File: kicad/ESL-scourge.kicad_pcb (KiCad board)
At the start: 2 copper layers, 80 x 50 mm, 41 parts, among them IC1 MOC3020M, J1 DB9, J2 DB9, P1 CONN_4, P2 CONN_3, P3 CONN_4, Q1 BC847, Q2 BC847, Q3 BC847, U1 TDA2030

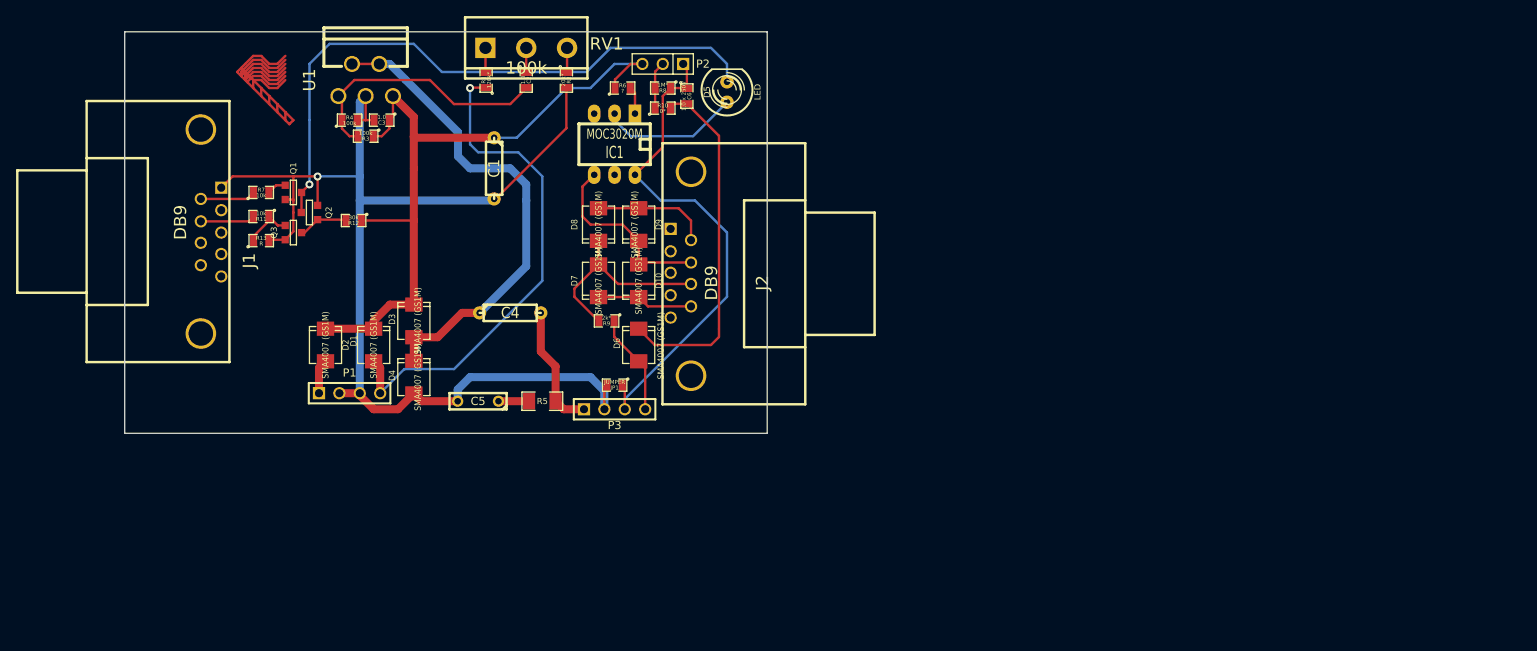
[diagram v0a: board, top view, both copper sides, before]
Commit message: Add initial maket_lovat as a separate branch (kicad folder only)
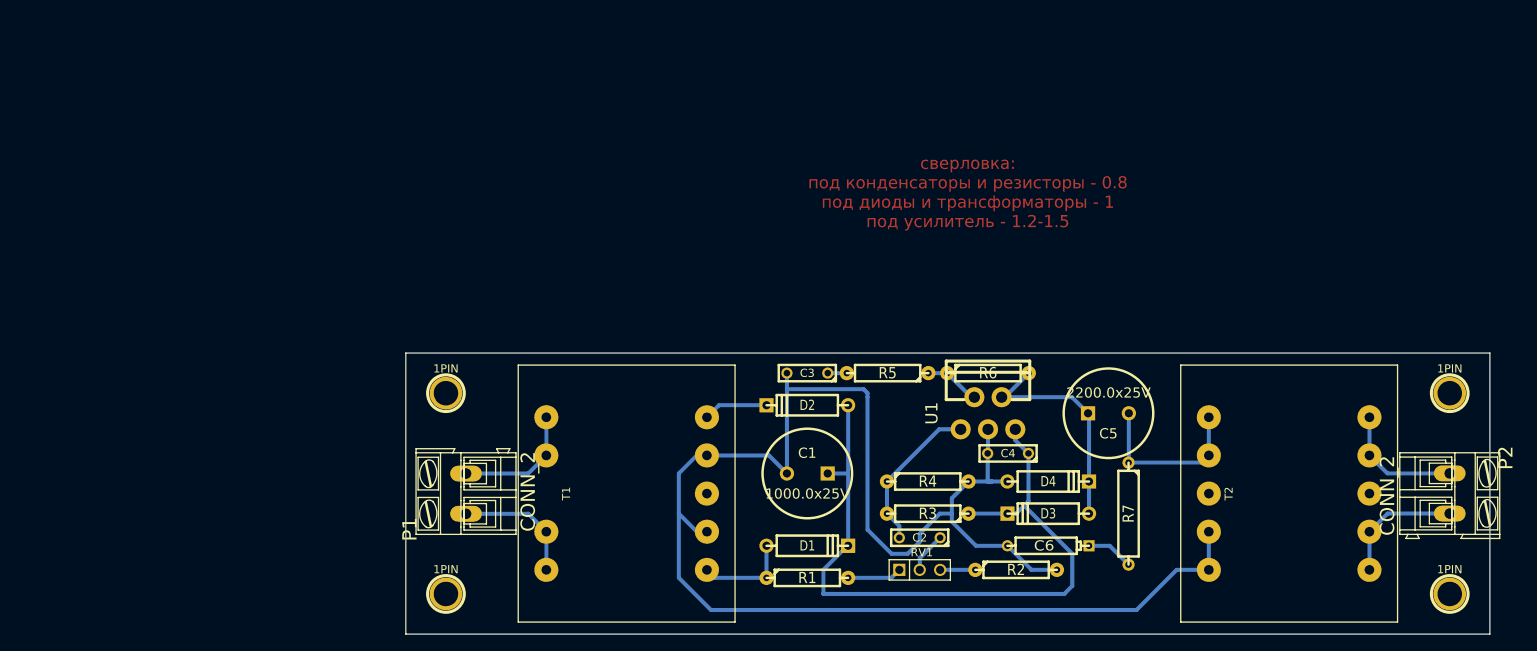
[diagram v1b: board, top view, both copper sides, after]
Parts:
- removed D10, D6, D7, D8, D9: SMA4007 (GS1M), DO_214AA
- removed D5: LED, LED-5MM
- removed IC1: MOC3020M, DIP-6__300_ELL
- removed J1: DB9, DB9MC
- removed J2: DB9, DB9FC
- removed JP1: JUMPER, SM0805
- removed P3: CONN_4, PIN_ARRAY_4x1
- removed Q1, Q2, Q3: BC847, SOT23EBC
- removed R10: 0*, SM0805
- removed R11: 10k, SM0805
- removed R12: 30k, SM0805
- removed R13: R, SM0805
- removed R8: 1M*, SM0805
- removed R9: 2k*, SM0805
- added 1PIN: P***, 1pin, F.Cu at (165.0, 45.0)
- added 1PIN: P***, 1pin, F.Cu at (165.0, 70.0)
- added 1PIN: P***, 1pin, F.Cu at (40.0, 45.0)
- added 1PIN: P***, 1pin, F.Cu at (40.0, 70.0)
- added T1: ТПК-1 (2х9В, 0.08А) (ТПГ-1), TPG-1, F.Cu at (62.5, 57.5)
- added T2: ТПК-1 (18В, 0.08А) (ТПГ-1), TPG-1, F.Cu at (145.0, 57.5)
- C1: footprint R3-LARGE_PADS -> C2V10
- C2, C3: footprint SM0805 -> C2
- C4: value 2200.0x25V -> 1.0; footprint R3-LARGE_PADS -> C2
- C5: value 0.22 -> 2200.0x25V; footprint C2 -> C2V10
- C6: value 1.0 x 250V -> 0.22; footprint SM0805 -> CP4
- D1, D2, D3, D4: value SMA4007 (GS1M) -> DIODE; footprint DO_214AA -> D4
- P1: value CONN_4 -> CONN_2; footprint PIN_ARRAY_4x1 -> AK300-2
- P2: value CONN_3 -> CONN_2; footprint PIN_ARRAY_3X1 -> AK300-2
- R1, R2, R3, R4: footprint SM0805 -> R4-LARGE_PADS
- R5: value 1 -> 100k; footprint SM1206 -> R4-LARGE_PADS
- R6: value ? -> 100k; footprint SM0805 -> R4-LARGE_PADS
- R7: value 10k -> 1; footprint SM0805 -> R5
- RV1: footprint bornier3 -> PIN_ARRAY_3X1
- moved R7 115.2 mm to (125.0, 60.0), turned to 270 degrees
- moved P2 111.7 mm to (165.0, 57.5), turned to 270 degrees
- moved U1 87.9 mm to (107.5, 47.5)
- moved R4 84.9 mm to (100.0, 56.0)
- moved R3 84.3 mm to (100.0, 60.0)
- moved R2 82.8 mm to (111.0, 67.0), turned to 0 degrees
- moved D3 82.6 mm to (115.0, 60.0), turned to 180 degrees
- moved RV1 81.4 mm to (99.0, 67.0)
- moved D4 80.1 mm to (115.0, 56.0), turned to 0 degrees
- moved C5 78.5 mm to (122.5, 47.5), turned to 0 degrees
- moved C2 75.2 mm to (99.0, 63.0), turned to 180 degrees
- moved R1 73.8 mm to (85.0, 68.0), turned to 0 degrees
- moved C6 71.8 mm to (115.0, 64.0), turned to 180 degrees
- moved C4 64.4 mm to (110.0, 52.5), turned to 180 degrees
- moved C3 61.7 mm to (85.0, 42.5)
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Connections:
- C1 pad 1: VCC -> N-0000016
- C3 pad 1: VCC -> N-0000010
- C4 pad 1: N-000005 -> N-0000016
- C4 pad 2: N-0000024 -> GND
- C5 pad 1: N-000007 -> N-0000013
- C5 pad 2: GND -> N-0000014
- C6 pad 1: N-0000025 -> N-0000012
- C6 pad 2: N-0000023 -> GND
- D1 pad 1: N-0000011 -> N-000007
- D1 pad 2: VCC -> N-0000016
- D2 pad 1: N-0000013 -> N-0000016
- D2 pad 2: VCC -> N-000003
- D3 pad 1: N-000005 -> N-0000013
- D3 pad 2: VCC -> N-0000016
- D4 pad 2: N-000005 -> N-0000013
- P1 pad 1: N-0000013 -> N-000004
- P1 pad 2: GND -> N-000005
- P2 pad 1: N-0000025 -> N-000001
- R1 pad 1: N-0000011 -> N-000007
- R3 pad 1: VCC -> N-0000016
- R5 pad 1: N-0000024 -> N-0000015
- R5 pad 2: N-000007 -> N-0000010
- R6 pad 1: VCC -> N-0000015
- R6 pad 2: N-0000018 -> N-0000013
- R7 pad 1: N-0000021 -> N-0000014
- R7 pad 2: N-0000022 -> N-0000012
- U1 pad 2: N-000005 -> N-0000015
- U1 pad 4: N-000005 -> N-0000013
- U1 pad 5: VCC -> N-0000016
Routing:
- net VCC: track 90.8 -> 0.00 mm
- net N-0000016: track 6.28 -> 89.0 mm
- net N-000006 (its old number): track 77.7 -> 0.00 mm, vias 1 -> 0
- net (no net): track 70.4 -> 0.00 mm
- net N-0000011: track 63.0 -> 0.00 mm, vias 1 -> 0
- net N-0000025: track 62.8 -> 0.00 mm
- net N-000005: track 60.5 -> 15.7 mm
- net N-0000023: track 44.3 -> 0.00 mm
- net GND: track 153.3 -> 194.7 mm, vias 1 -> 0
- net N-0000013: track 4.30 -> 28.8 mm
- net N-0000032: track 23.6 -> 0.00 mm
- net N-0000019: track 17.4 -> 0.00 mm
- net N-0000024: track 15.7 -> 0.00 mm
- net N-000004: track 0.00 -> 15.7 mm
- net N-0000014: track 6.24 -> 21.3 mm
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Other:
- board size 80 x 50 mm -> 135 x 35 mm
- net class Default: clearance 0.3 -> 0.5; trace_width 0.3 -> 0.5
- rule trace_clearance: 0.3 -> 0.5
- board text added: "сверловка: под конденсаторы и резисторы - 0.8 под диоды и трансформаторы - 1 под усилитель - 1.2-1.5"
